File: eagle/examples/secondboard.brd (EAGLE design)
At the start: 16.5 x 25.1 mm, 3 parts

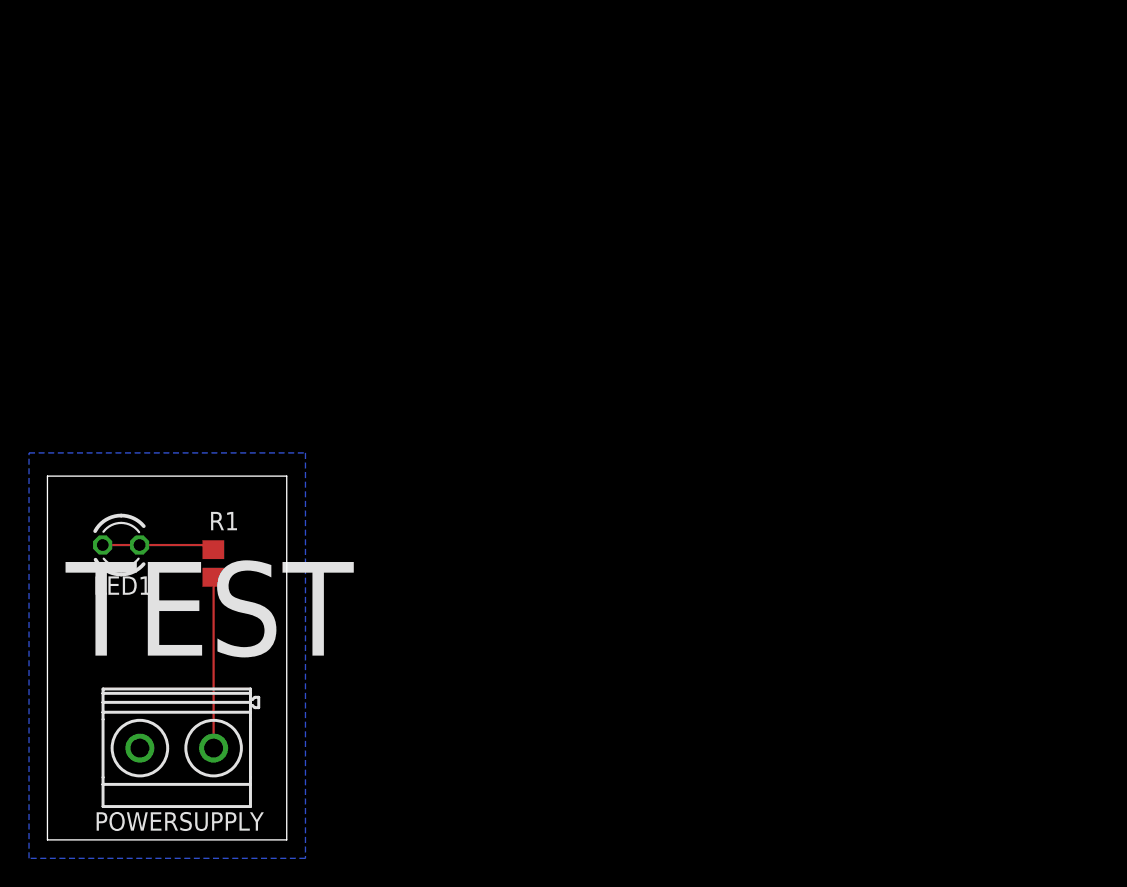
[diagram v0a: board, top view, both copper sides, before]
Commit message: examples
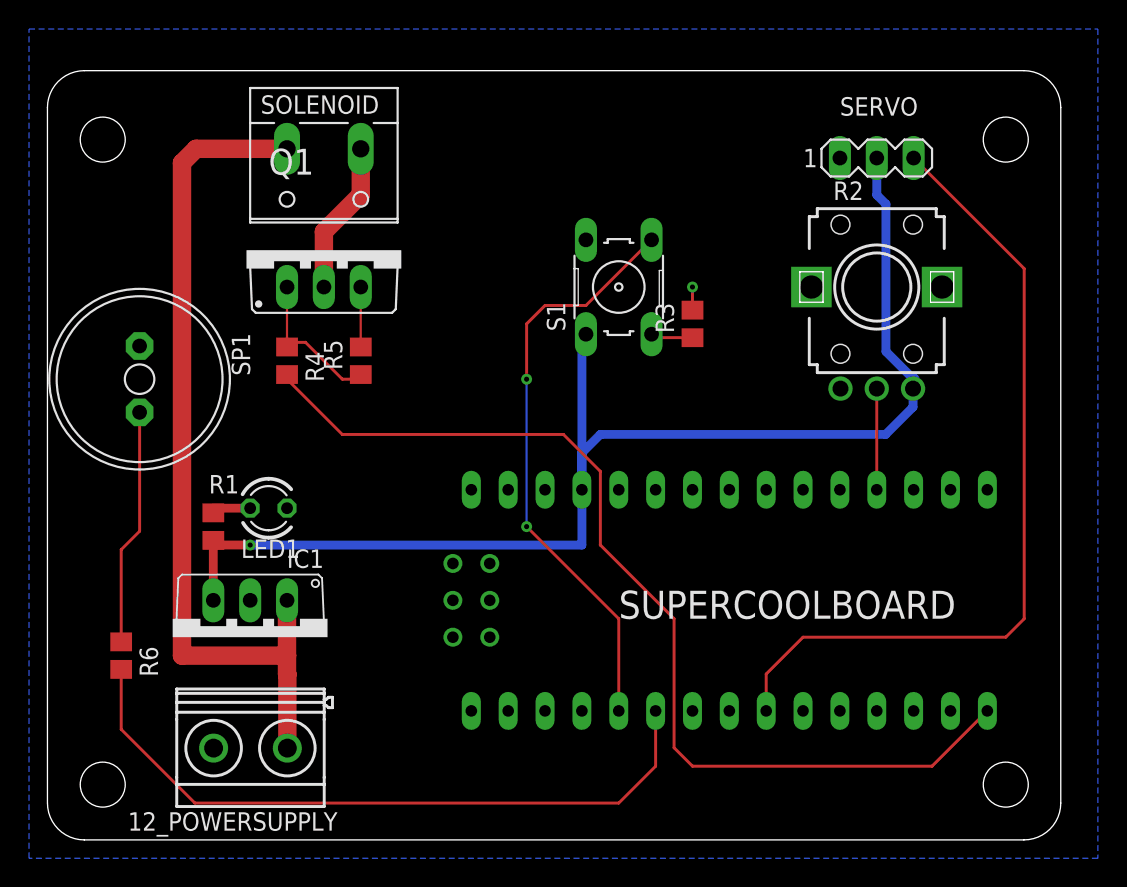
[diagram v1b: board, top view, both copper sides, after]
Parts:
- removed POWERSUPPLY: MKDSN1,5/2-5,08, con-phoenix-508:MKDSN1,5/2-5,08
- added 12_POWERSUPPLY: MKDSN1,5/2-5,08, con-phoenix-508:MKDSN1,5/2-5,08
- added IC1: 7805TV, linear:TO220V
- added Q1: IRF540, transistor-power:TO220BV
- added R2: EVUF3A, pot:EVUF
- added R3: 10K, rcl:R0805
- added R4: 1K, rcl:R0805
- added R5: 100K, rcl:R0805
- added R6: 100, rcl:R0805
- added S1: (no value), switch-omron:B3F-10XX
- added SERVO: (no value), con-lstb:MA03-1
- added SOLENOID: (no value), con-wago-508:W237-132
- added SP1: AL11P, buzzer:AL11P
- added U$1: NANO, Arduino-clone:NANO
- moved LED1 10.5 mm to (15.2, 22.9)
- moved R1 2.54 mm to (11.4, 21.6)
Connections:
- new net +12V: 12_POWERSUPPLY.1, IC1.1, SOLENOID.2
- new net BUTTON: S1.4, U$1.D2
- new net BUZZ: R6.2, U$1.D3
- new net MOSFET: R4.2, U$1.D12
- new net N$1: R3.1, S1.3
- new net N$2: R6.1, SP1.+
- new net N$3: Q1.D, SOLENOID.1
- new net N$4: SERVO.3, U$1.D6
- new net N$6: Q1.G, R4.1, R5.1
- new net POT_OUT: R2.2, U$1.A0
- net +5V: now also IC1.3, R2.3, S1.1, SERVO.2, U$1.5V; no longer POWERSUPPLY.1
- net GND: now also 12_POWERSUPPLY.2, IC1.2, Q1.S, R2.1, R3.2, R5.2, SERVO.1, SP1.-, U$1.GND; no longer POWERSUPPLY.2
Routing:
- net +5V: track 11.8 -> 89.2 mm, vias 0 -> 1
- net MOSFET: track 0.00 -> 69.4 mm
- net +12V: track 0.00 -> 59.0 mm
- net N$4: track 0.00 -> 56.8 mm
- net BUZZ: track 0.00 -> 47.9 mm
- net BUTTON: track 0.00 -> 40.3 mm, vias 0 -> 2
- net N$2: track 0.00 -> 16.3 mm
- net N$3: track 0.00 -> 10.6 mm
- net N$6: track 0.00 -> 10.4 mm
- net POT_OUT: track 0.00 -> 6.97 mm
- net GND: track 0.00 -> 5.72 mm, vias 0 -> 1
- net CONNECT: track 7.75 -> 2.86 mm
- net N$1: track 0.00 -> 2.92 mm
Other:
- board size 16.5 x 25.1 mm -> 69.8 x 53 mm
- board text added: "SUPERCOOLBOARD"
- board text removed: "TEST"
